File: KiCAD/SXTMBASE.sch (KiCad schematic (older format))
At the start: 97 parts

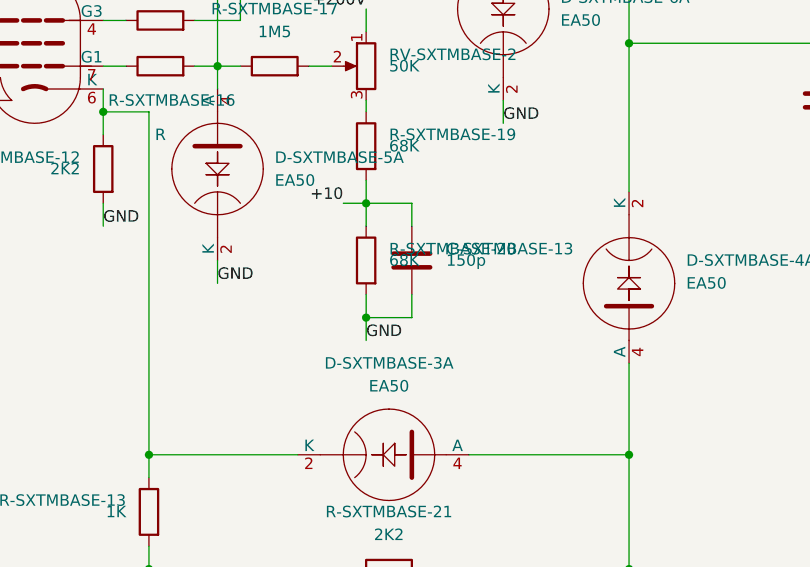
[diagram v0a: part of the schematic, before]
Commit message: Add TYPEWE WRERCCTS YAMP&HVR.
Which com,pletes the first pass. All the pages are done but I haven't checked them yet and there are bound to be errosr.

Signed-off-by: John Bradley <flypie@rocketmail.com>
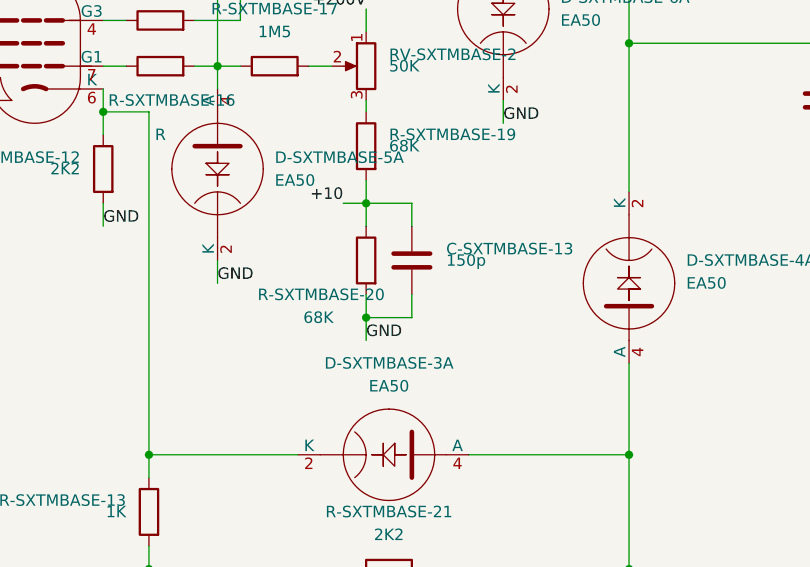
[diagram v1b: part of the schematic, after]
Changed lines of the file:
@@
 $Descr A3 16535 11693
 encoding utf-8
-Sheet 41 42
+Sheet 41 45
 Title "Dot and Strobe 2.3"
 Date "2020-10-15"
@@
 U 1 1 60681CD8
 P 4925 3550
-F 0 "R-SXTMBASE-20" H 4825 3600 50  0000 R CNN
-F 1 "68K" H 4825 3550 50  0000 R CNN
+F 0 "R-SXTMBASE-20" H 5400 3400 50  0000 R CNN
+F 1 "68K" H 5200 3300 50  0000 R CNN
 F 2 "Resistor_THT:R_Axial_DIN0516_L15.5mm_D5.0mm_P5.08mm_Vertical" V 4855 3550 50  0001 C CNN
 F 3 "~" H 4925 3550 50  0001 C CNN
